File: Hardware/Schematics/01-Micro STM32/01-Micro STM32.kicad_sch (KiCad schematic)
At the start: 24 parts, among them J1 Screw_Terminal_01x04, J2 Conn_01x12_MountingPin, J3 Conn_02x25_Odd_Even, SW1 SW_DIP_x05, U1 MCP23017_ML, U2 ESP32-DEVKITC-32D, U3 74HCT138, U4 74HCT138, U5 CP2102N-Axx-xQFN28, U6 USBLC6-2SC6, U69A AD8604ARUZ

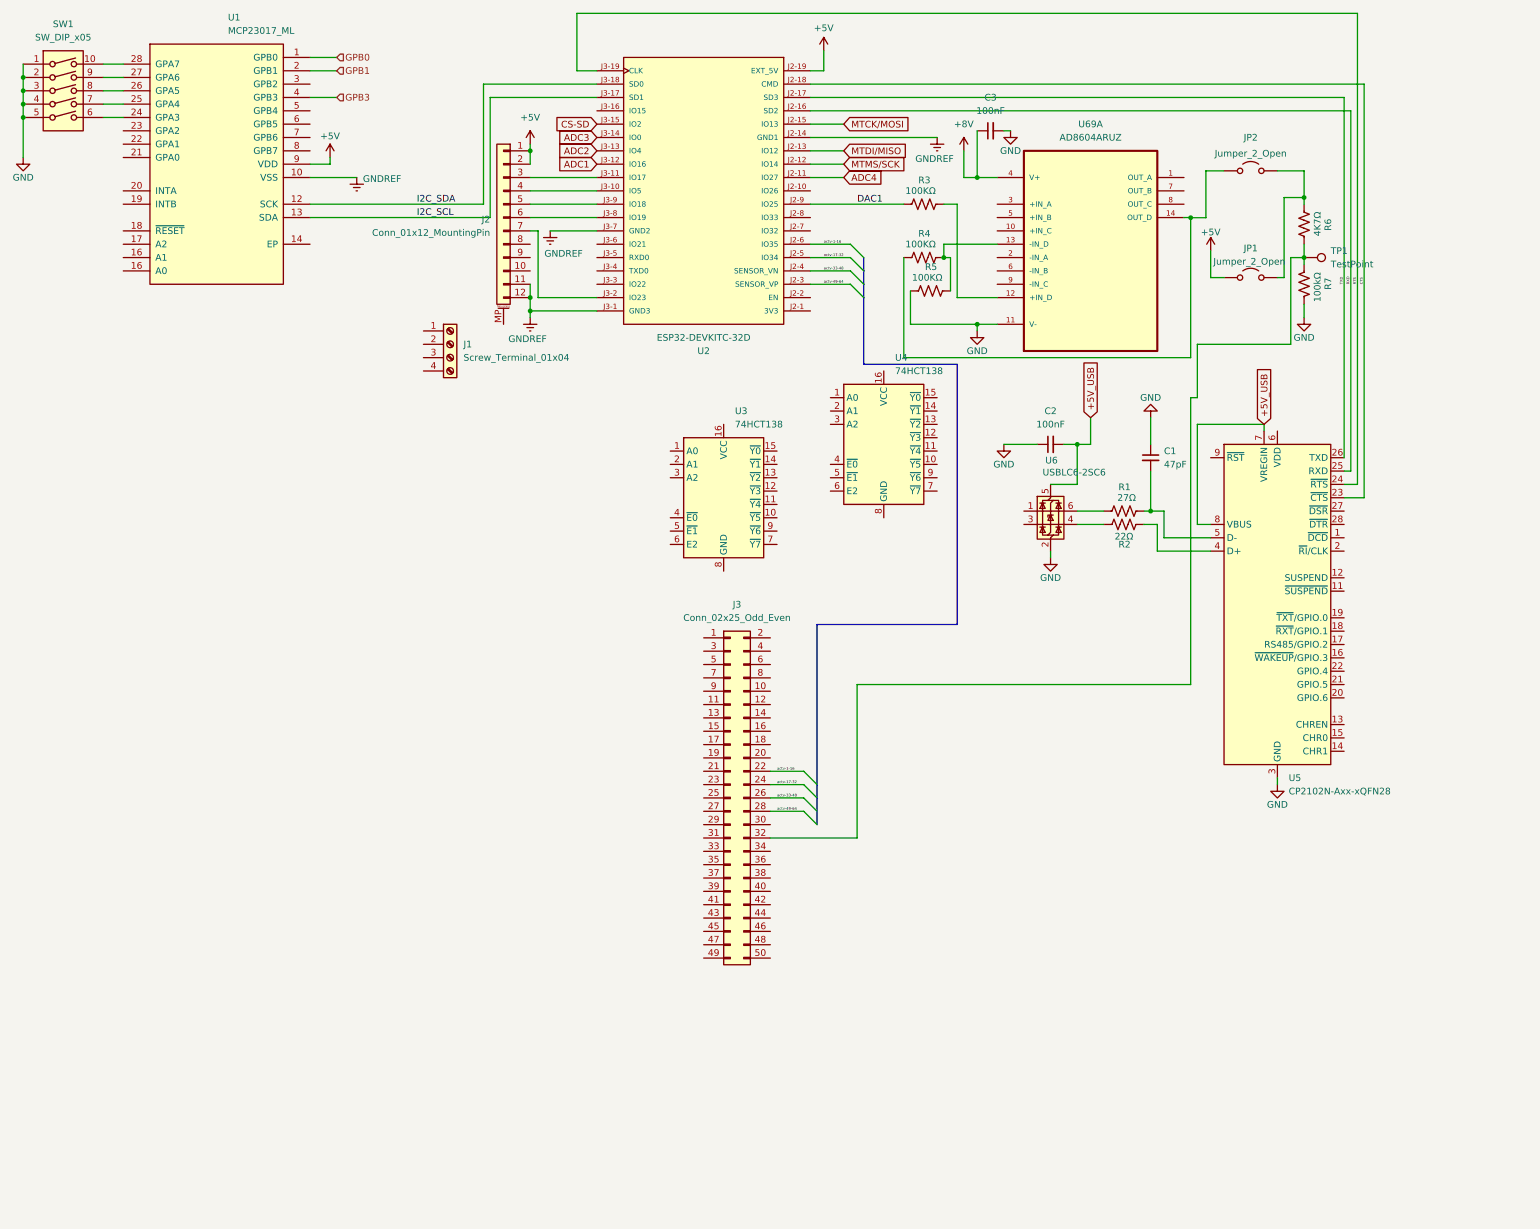
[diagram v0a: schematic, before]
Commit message: update
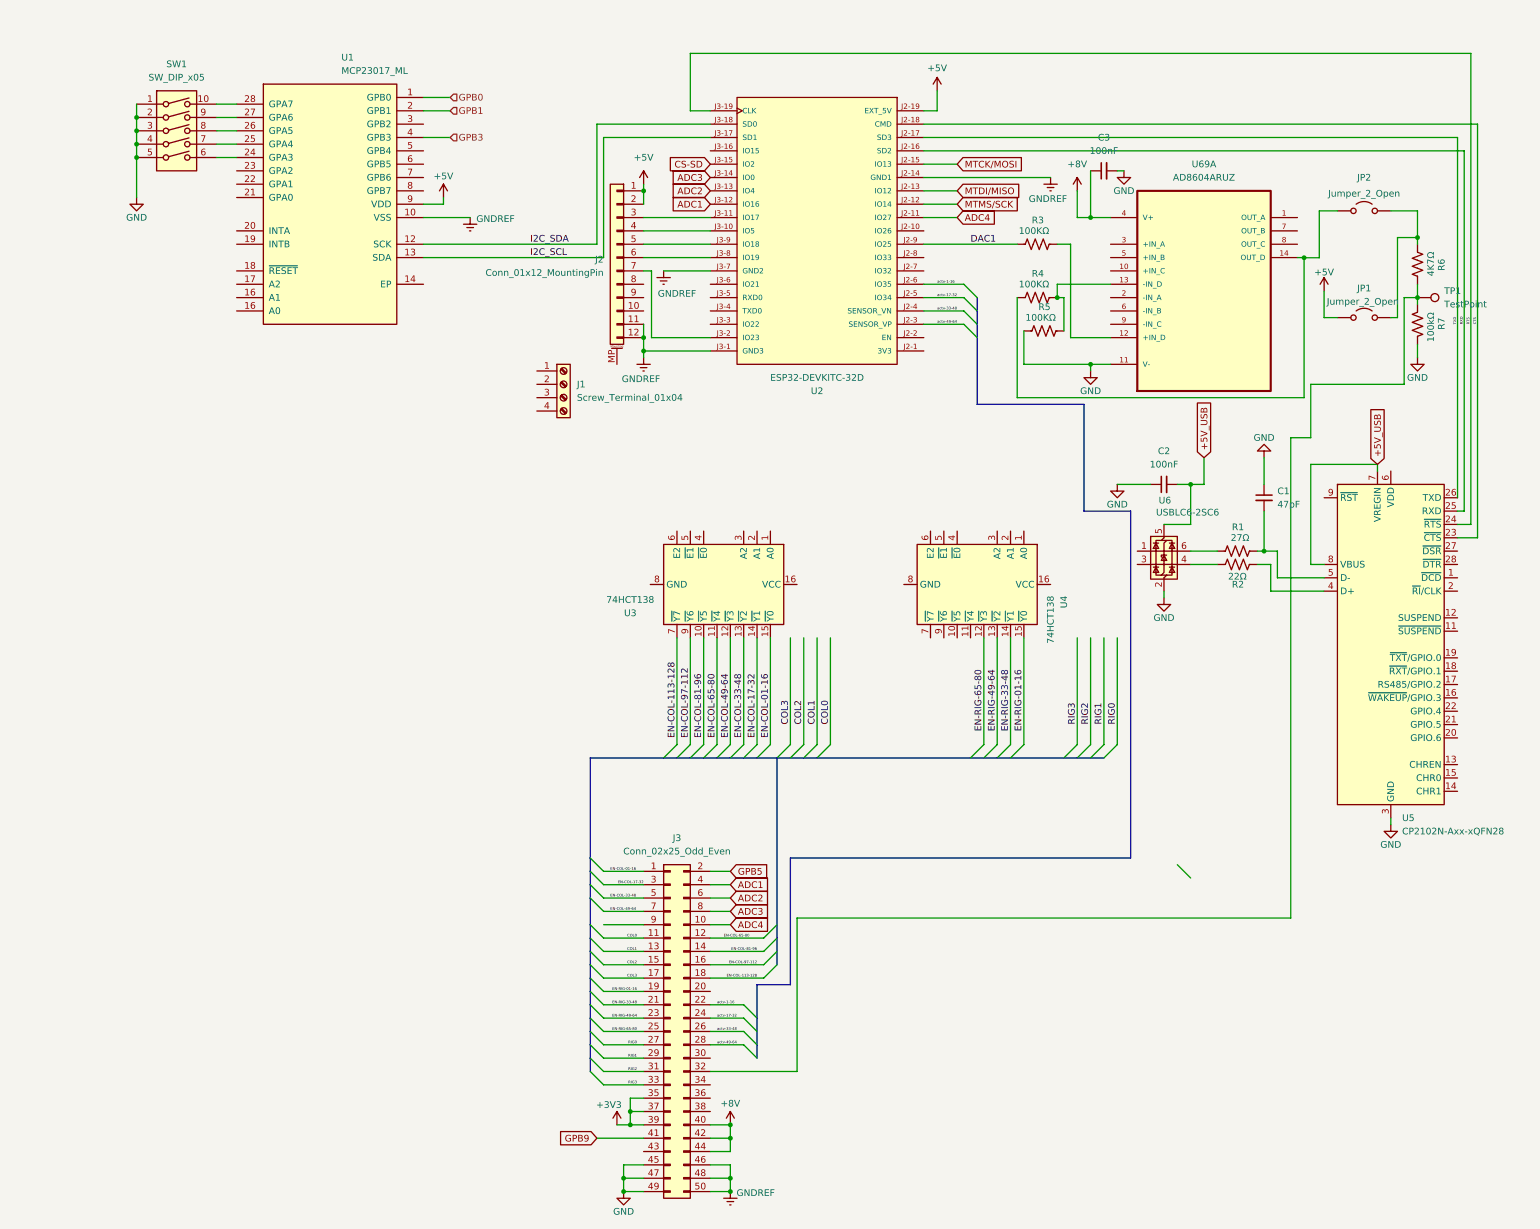
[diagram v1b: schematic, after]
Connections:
- net +8V: now also J3.40 (Pin_40), J3.42 (Pin_42), J3.44 (Pin_44)
- net ADC1: now also J3.4 (Pin_4)
- net ADC2: now also J3.6 (Pin_6)
- net ADC3: now also J3.8 (Pin_8)
- net ADC4: now also J3.10 (Pin_10)
- net GND: now also J3.45 (Pin_45), J3.47 (Pin_47), J3.49 (Pin_49)
- net GNDREF: now also J3.46 (Pin_46), J3.48 (Pin_48), J3.50 (Pin_50)
- net EN-RIG-65-80: now reaches U4.12 (~{Y3})
- net EN-RIG-65-80: now also J3.25 (Pin_25)
- net EN-RIG-49-64: now reaches U4.13 (~{Y2})
- net EN-RIG-49-64: now also J3.23 (Pin_23)
- net EN-RIG-33-48: now reaches U4.14 (~{Y1})
- net EN-RIG-33-48: now also J3.21 (Pin_21)
- net EN-RIG-01-16: now reaches U4.15 (~{Y0})
- net EN-RIG-01-16: now also J3.19 (Pin_19)
- net EN-COL-01-16: now reaches J3.1 (Pin_1)
- net EN-COL-01-16: now also U3.15 (~{Y0})
- net COL0: now reaches J3.11 (Pin_11)
- net EN-COL-65-80: now reaches J3.12 (Pin_12)
- net EN-COL-65-80: now also U3.11 (~{Y4})
- net COL1: now reaches J3.13 (Pin_13)
- net EN-COL-81-96: now reaches J3.14 (Pin_14)
- net EN-COL-81-96: now also U3.10 (~{Y5})
- net COL2: now reaches J3.15 (Pin_15)
- net EN-COL-97-112: now reaches J3.16 (Pin_16)
- net EN-COL-97-112: now also U3.9 (~{Y6})
- net COL3: now reaches J3.17 (Pin_17)
- net EN-COL-113-128: now reaches J3.18 (Pin_18)
- net EN-COL-113-128: now also U3.7 (~{Y7})
- net GPB5: now reaches J3.2 (Pin_2)
- net RIG0: now reaches J3.27 (Pin_27)
- net RIG1: now reaches J3.29 (Pin_29)
- net EN-COL-17-32: now reaches J3.3 (Pin_3)
- net EN-COL-17-32: now also U3.14 (~{Y1})
- net RIG2: now reaches J3.31 (Pin_31)
- net RIG3: now reaches J3.33 (Pin_33)
- net +3V3: now reaches J3.35 (Pin_35)
- net +3V3: now also J3.37 (Pin_37), J3.39 (Pin_39)
- net GPB9: now reaches J3.41 (Pin_41)
- net EN-COL-33-48: now reaches J3.5 (Pin_5)
- net EN-COL-33-48: now also U3.13 (~{Y2})
- net EN-COL-49-64: now reaches J3.7 (Pin_7)
- net EN-COL-49-64: now also U3.12 (~{Y3})
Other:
- moved on the sheet: C1, C2, C3, J1, J2, J3, JP1, JP2, R1, R2, R3, R4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
